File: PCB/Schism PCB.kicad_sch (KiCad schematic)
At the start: 106 parts, among them J1 USB C Connector, J2 JTAG_TC2030, J3 USB_C_Receptacle_USB2.0, J4 USB_C_Receptacle_USB2.0, J5 Conn_01x06_MountingPin, J6 Conn_01x06_MountingPin, J7 Conn_01x06_MountingPin, J8 Conn_01x06, J9 Conn_01x06, SW1 Boot, U1 XC6206, U2 USBLC6-2SC6, U3 RP2040, U4 W25Q128JVS, U5 MCP23017_SO, Y1 12MHz

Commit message: Pre-production files v0.3
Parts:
- added C13: 100nF, Capacitor_SMD:C_0402_1005Metric, symbol Device:C_Small
- added J10: Conn_01x04_MountingPin, Connector_JST:JST_SH_SM04B-SRSS-TB_1x04-1MP_P1.00mm_Horizontal, symbol Connector_Generic_MountingPin:Conn_01x04_MountingPin
- added J11: USB_A, Connector_USB:USB_A_Receptacle_GCT_USB1046, symbol Connector:USB_A
- added J12: Conn_01x04, Connector_PinHeader_2.54mm:PinHeader_1x04_P2.54mm_Vertical, symbol Connector_Generic:Conn_01x04
- added J13: Conn_01x10, Connector_PinHeader_2.54mm:PinHeader_1x10_P2.54mm_Vertical, symbol Connector_Generic:Conn_01x10
- added R1: 1M, Resistor_SMD:R_0603_1608Metric, symbol Device:R_Small
- added R7 (x3): 10k, Resistor_SMD:R_0402_1005Metric, symbol Device:R_Small
- J5: value Conn_01x06_MountingPin -> JST
- J6: value Conn_01x06_MountingPin -> JST Left
- J7: value Conn_01x06_MountingPin -> JST Right
- J8: value Conn_01x06 -> 2.54 Header
- J9: value Conn_01x06 -> 2.54
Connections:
- net +3V3: now also C13.2, J10.1 (Pin_1), J11.1 (VBUS), J12.4 (Pin_4), R7.1, R7.2, R7.2
- net A_2: now also J6.5 (Pin_5), J7.5 (Pin_5), J9.3 (Pin_3); no longer J6.3 (Pin_3), J7.3 (Pin_3)
- net C_DN_2: now also J6.6 (Pin_6), J7.6 (Pin_6), J9.2 (Pin_2); no longer J6.2 (Pin_2), J7.2 (Pin_2)
- net C_LT_2: now also J9.4 (Pin_4)
- net C_RT_2: now also J6.3 (Pin_3), J7.3 (Pin_3), J9.5 (Pin_5); no longer J6.5 (Pin_5), J7.5 (Pin_5)
- net C_UP_2: now also J6.2 (Pin_2), J7.2 (Pin_2), J9.6 (Pin_6); no longer J6.6 (Pin_6), J7.6 (Pin_6)
- net GND: now also U5.15 (A0), U5.16 (A1), U5.17 (A2), C13.1, J10.4 (Pin_4), J10.MP (MountPin), J11.4 (GND), J12.1 (Pin_1), J13.1 (Pin_1), R1.1
- net MS: now also U5.26 (GPA5); no longer U5.25 (GPA4)
- net SCL_2: now also R7.1
- net SDA_2: now also R7.2
- net Z: now also U5.25 (GPA4); no longer U5.26 (GPA5)
- net EX5: now reaches U3.11 (GPIO8)
- net EX5: now also J13.6 (Pin_6)
- net EX4: now reaches U3.15 (GPIO12)
- net EX4: now also J13.5 (Pin_5)
- net EX3: now reaches U3.16 (GPIO13)
- net EX3: now also J13.4 (Pin_4)
- net EX2: now reaches U3.17 (GPIO14)
- net EX2: now also J13.3 (Pin_3)
- net EX1: now reaches U3.18 (GPIO15)
- net EX1: now also J13.2 (Pin_2)
- net PD+: now reaches U3.27 (GPIO16)
- net PD+: now also J10.3 (Pin_3), J11.3 (D+), J12.2 (Pin_2)
- net PD-: now reaches U3.28 (GPIO17)
- net PD-: now also J10.2 (Pin_2), J11.2 (D-), J12.3 (Pin_3)
- net EX9: now reaches U3.6 (GPIO4)
- net EX9: now also J13.10 (Pin_10)
- net EX8: now reaches U3.7 (GPIO5)
- net EX8: now also J13.9 (Pin_9)
- net EX7: now reaches U3.8 (GPIO6)
- net EX7: now also J13.8 (Pin_8)
- net EX6: now reaches U3.9 (GPIO7)
- net EX6: now also J13.7 (Pin_7)
- net at U5.18 (~{RESET}): now also R7.1
- new net: J11.5 (Shield), R1.2
- no-connect marks 13 -> 18
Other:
- note added: "Buttons"
- note added: "C PAD"
- note added: "Connectors"
- note added: "LEFT HAND"
- note added: "Logos and Mousebites"
- note added: "RIGHT HAND"
- note added: "USB C i2c port"
- note added: "i2c chip"
- moved on the sheet: D2, D3, J3, J4, J5, J6, J7, J8, J9, MB5, MB6, MX1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

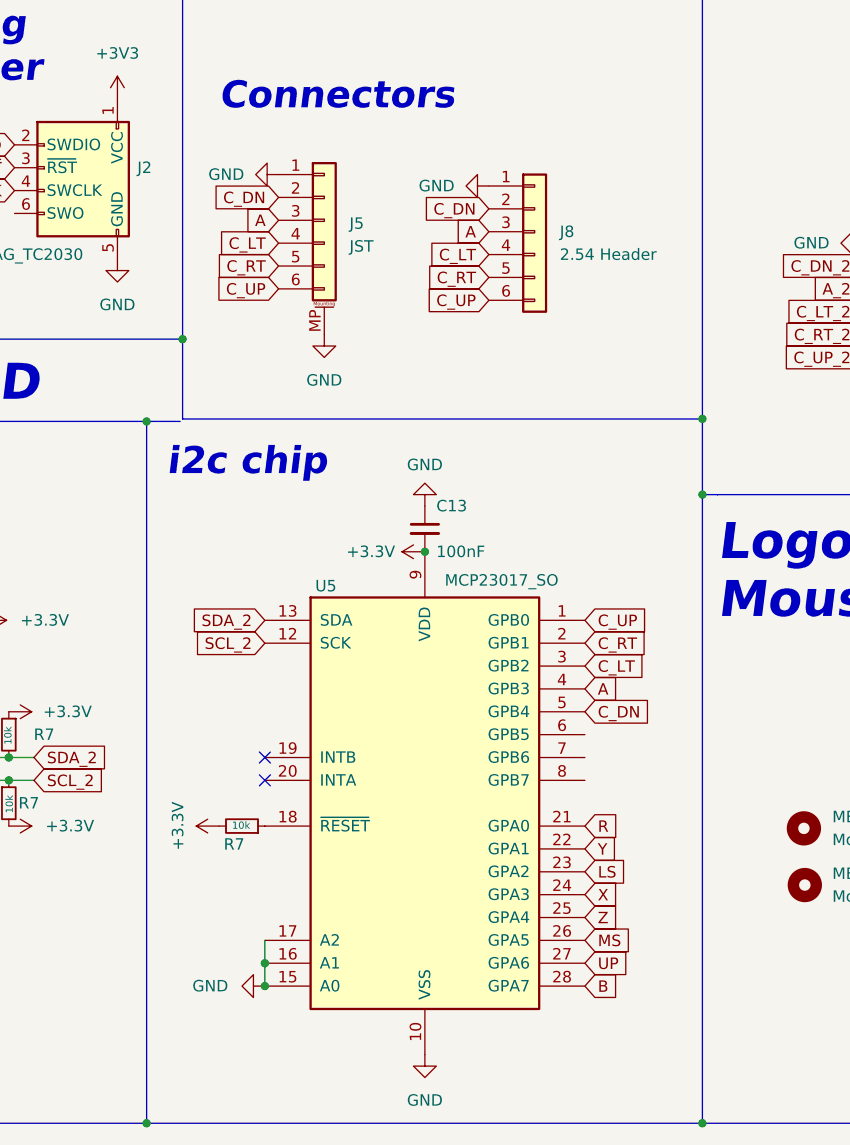
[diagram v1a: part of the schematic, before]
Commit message: v0.5
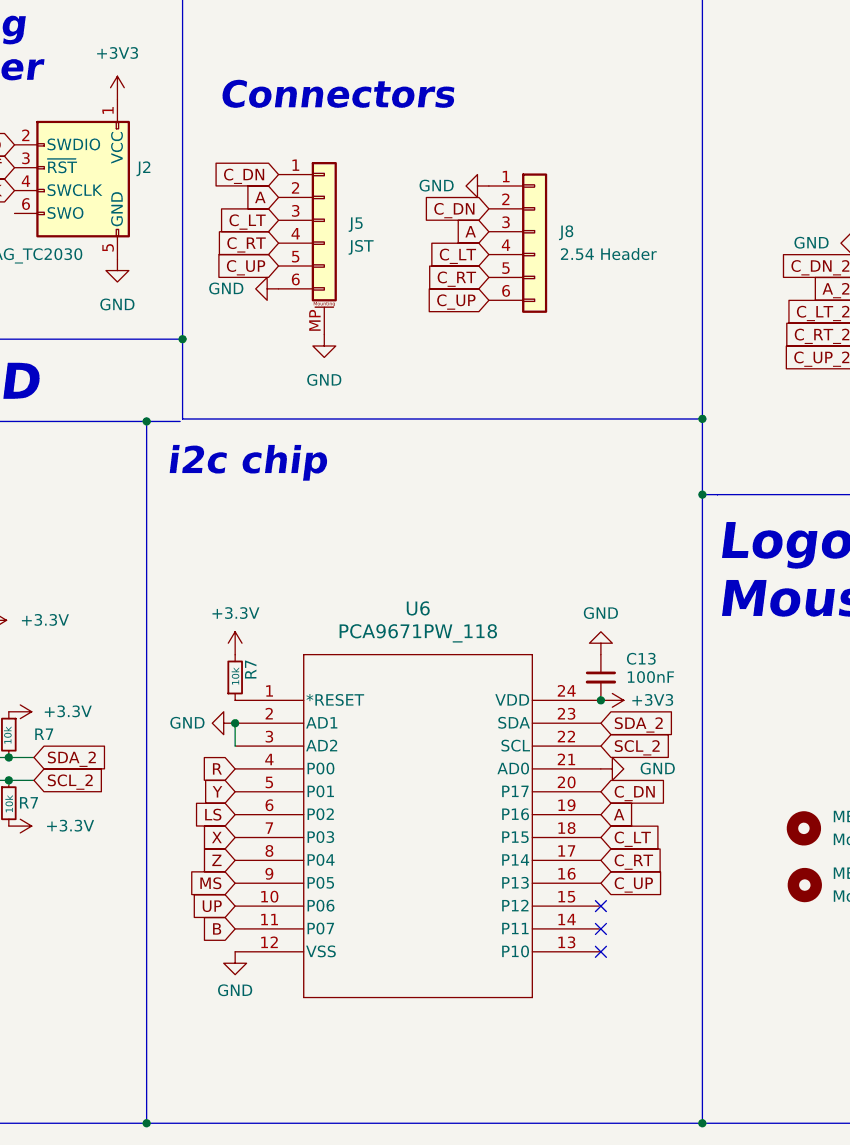
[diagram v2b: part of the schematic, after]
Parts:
- removed U5: MCP23017_SO, Package_SO:SOIC-28W_7.5x17.9mm_P1.27mm, symbol Interface_Expansion:MCP23017_SO
- added U6: PCA9671PW_118, TSSOP24_SOT355-1_NXP, symbol PCA9671PW:PCA9671PW_118
- J10, J11, J13, MB5, MB6: now left out of the parts list
- J3, J4: LCSC (none) -> C165948
- J5, J6, J7: LCSC (none) -> C160405
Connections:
- net +3V3: now also U6.24 (VDD)
- net A: now also J5.2 (Pin_2), U6.19 (P16); no longer J5.3 (Pin_3)
- net B: now also U6.11 (P07)
- net C_DN: now also J5.1 (Pin_1), U6.20 (P17); no longer J5.2 (Pin_2)
- net C_LT: now also J5.3 (Pin_3), U6.18 (P15); no longer J5.4 (Pin_4)
- net C_RT: now also J5.4 (Pin_4), U6.17 (P14); no longer J5.5 (Pin_5)
- net C_UP: now also J5.5 (Pin_5), U6.16 (P13); no longer J5.6 (Pin_6)
- net GND: now also J5.6 (Pin_6), U6.12 (VSS), U6.2 (AD1), U6.21 (AD0), U6.3 (AD2); no longer J5.1 (Pin_1)
- net LS: now also U6.6 (P02)
- net MS: now also U6.9 (P05)
- net R: now also U6.4 (P00)
- net SCL_2: now also U6.22 (SCL)
- net SDA_2: now also U6.23 (SDA)
- net UP: now also U6.10 (P06)
- net X: now also U6.7 (P03)
- net Y: now also U6.5 (P01)
- net Z: now also U6.8 (P04)
- net at R7.1: now also U6.1 (*RESET)
- no-connect marks 18 -> 19
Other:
- moved on the sheet: C13, R7
